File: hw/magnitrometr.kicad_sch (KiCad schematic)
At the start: 0 parts

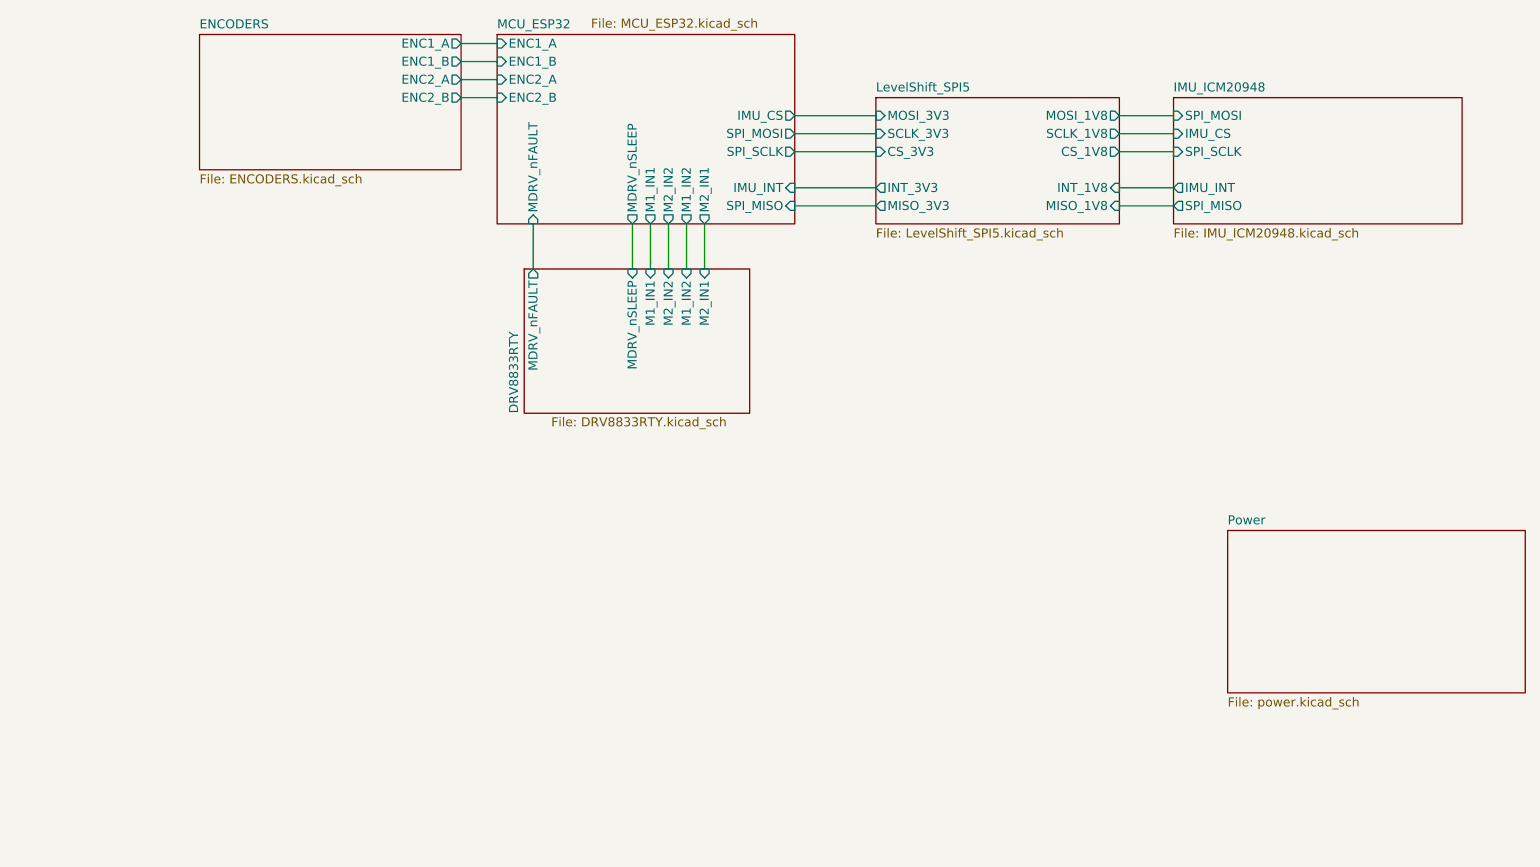
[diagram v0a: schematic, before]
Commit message: WIP
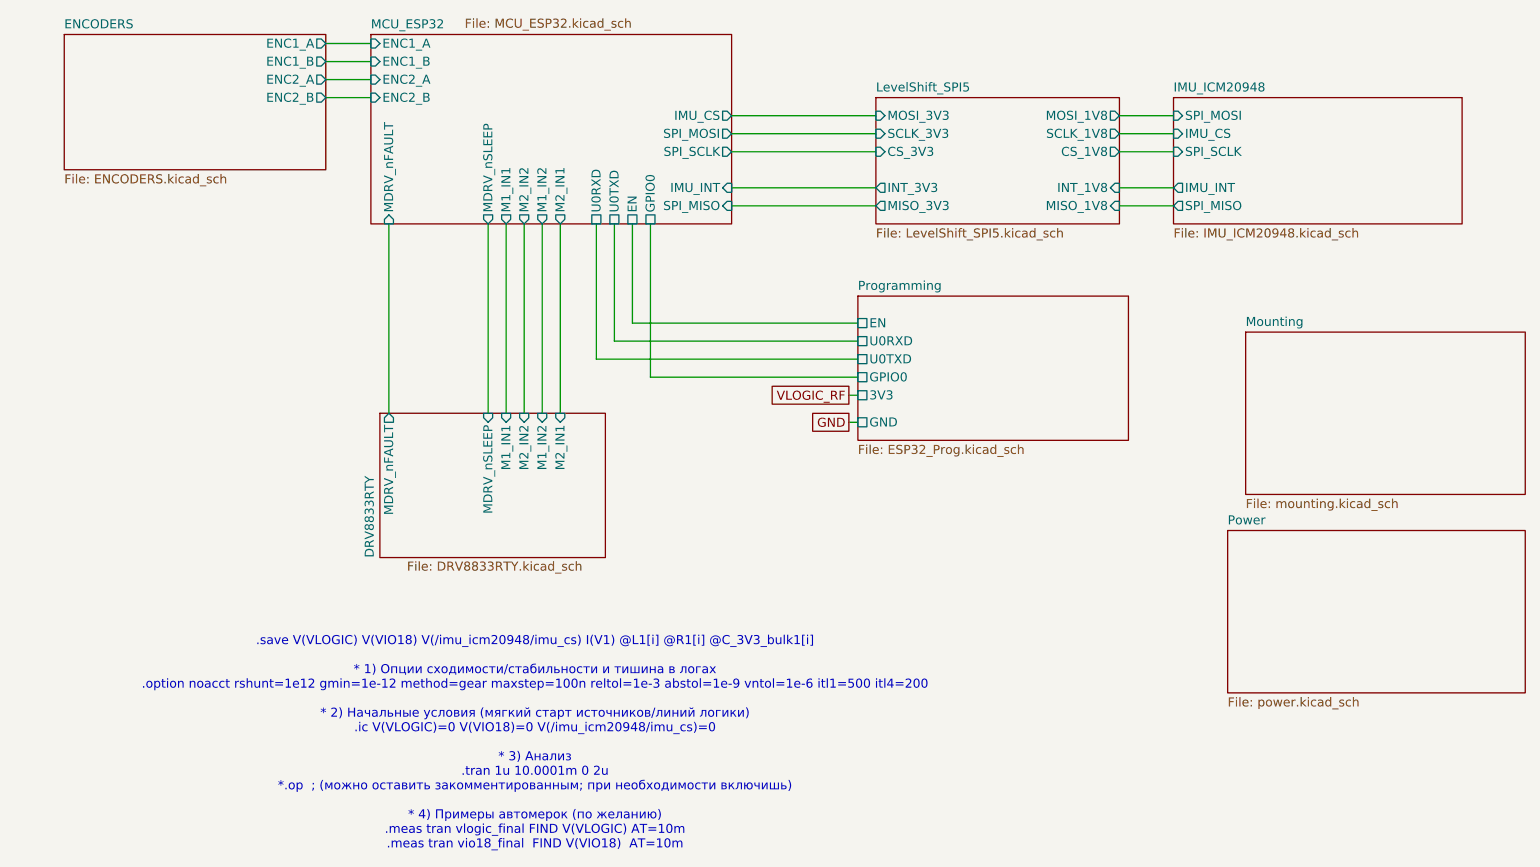
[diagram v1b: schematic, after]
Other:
- added sheet Mounting (mounting.kicad_sch)
- added sheet Programming (ESP32_Prog.kicad_sch)
- sheet MCU_ESP32 ports: added EN, GPIO0, U0RXD, U0TXD; removed none
- note added: ".save V(VLOGIC) V(VIO18) V(/imu_icm20948/imu_cs) I(V1) @L1[i] @R1[i] @C_3V3_bulk1[i] * 1) Опции сходимости/стабильности и тишина в логах .option noacct rshunt=1e12 gmin=1e-12 method=gear maxstep=100n reltol=1e-3 abstol=1e-9 vntol=1e-6 itl1=500 itl4=200 * 2) Начальные условия (мягкий старт источников/линий логики) .ic V(VLOGIC)=0 V(VIO18)=0 V(/imu_icm20948/imu_cs)=0 * 3) Анализ .tran 1u 10.0001m 0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"
